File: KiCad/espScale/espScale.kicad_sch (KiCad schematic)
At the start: 7 parts, among them U1 NodeMCU1.0(ESP-12E), U2 3-wire_Load_Cell, U4 3-wire_Load_Cell, U6 HX711_Load_Cell_Amplifier

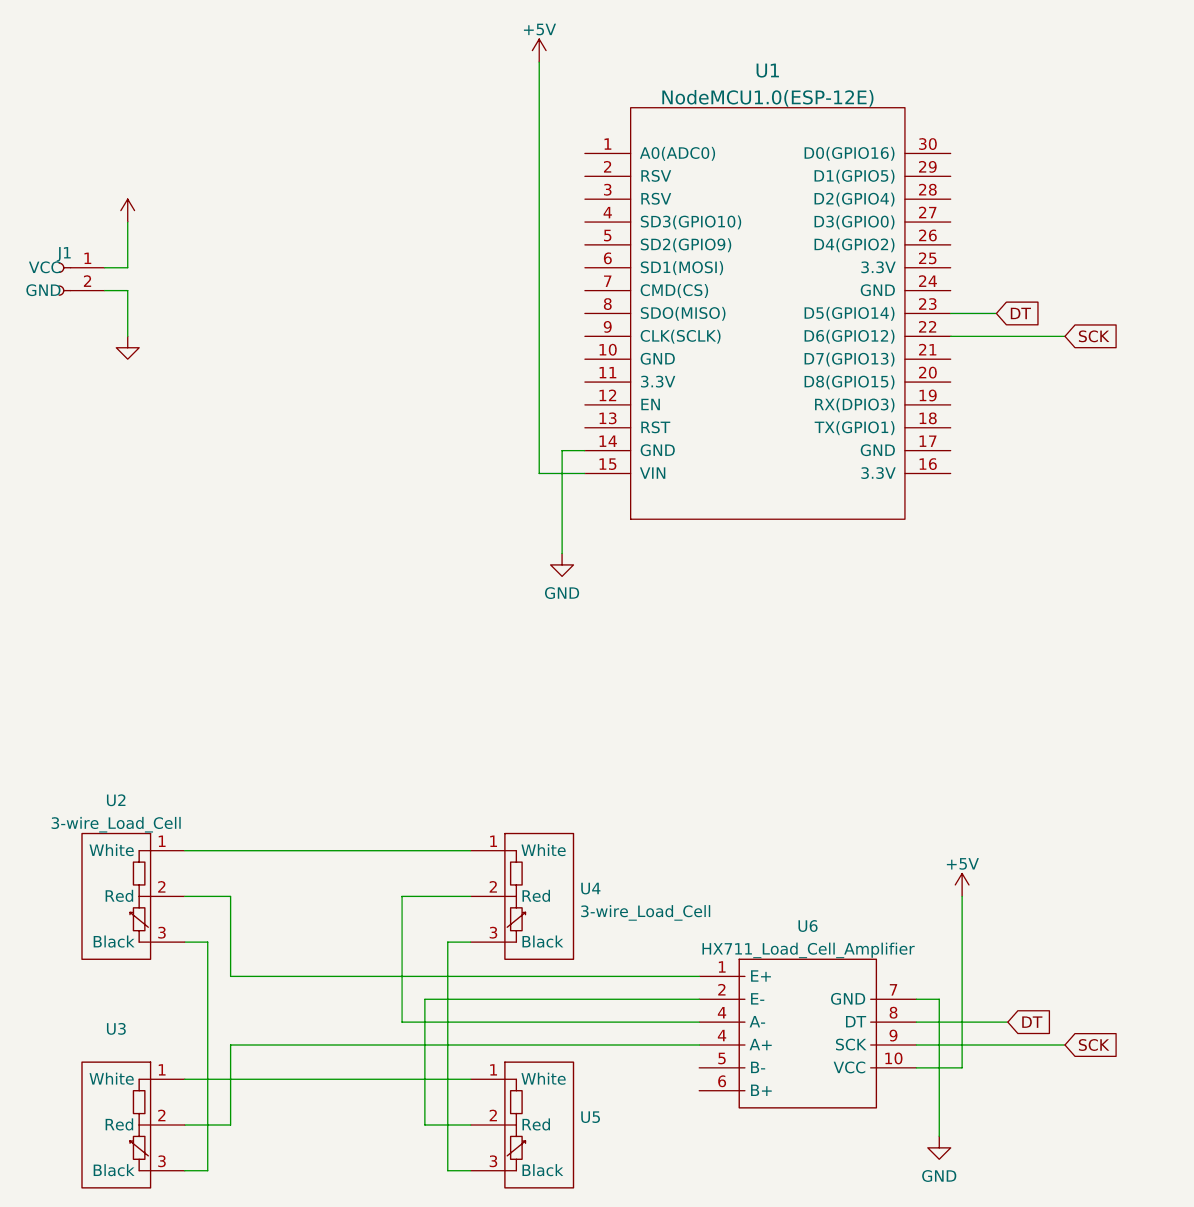
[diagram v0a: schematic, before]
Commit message: kicad
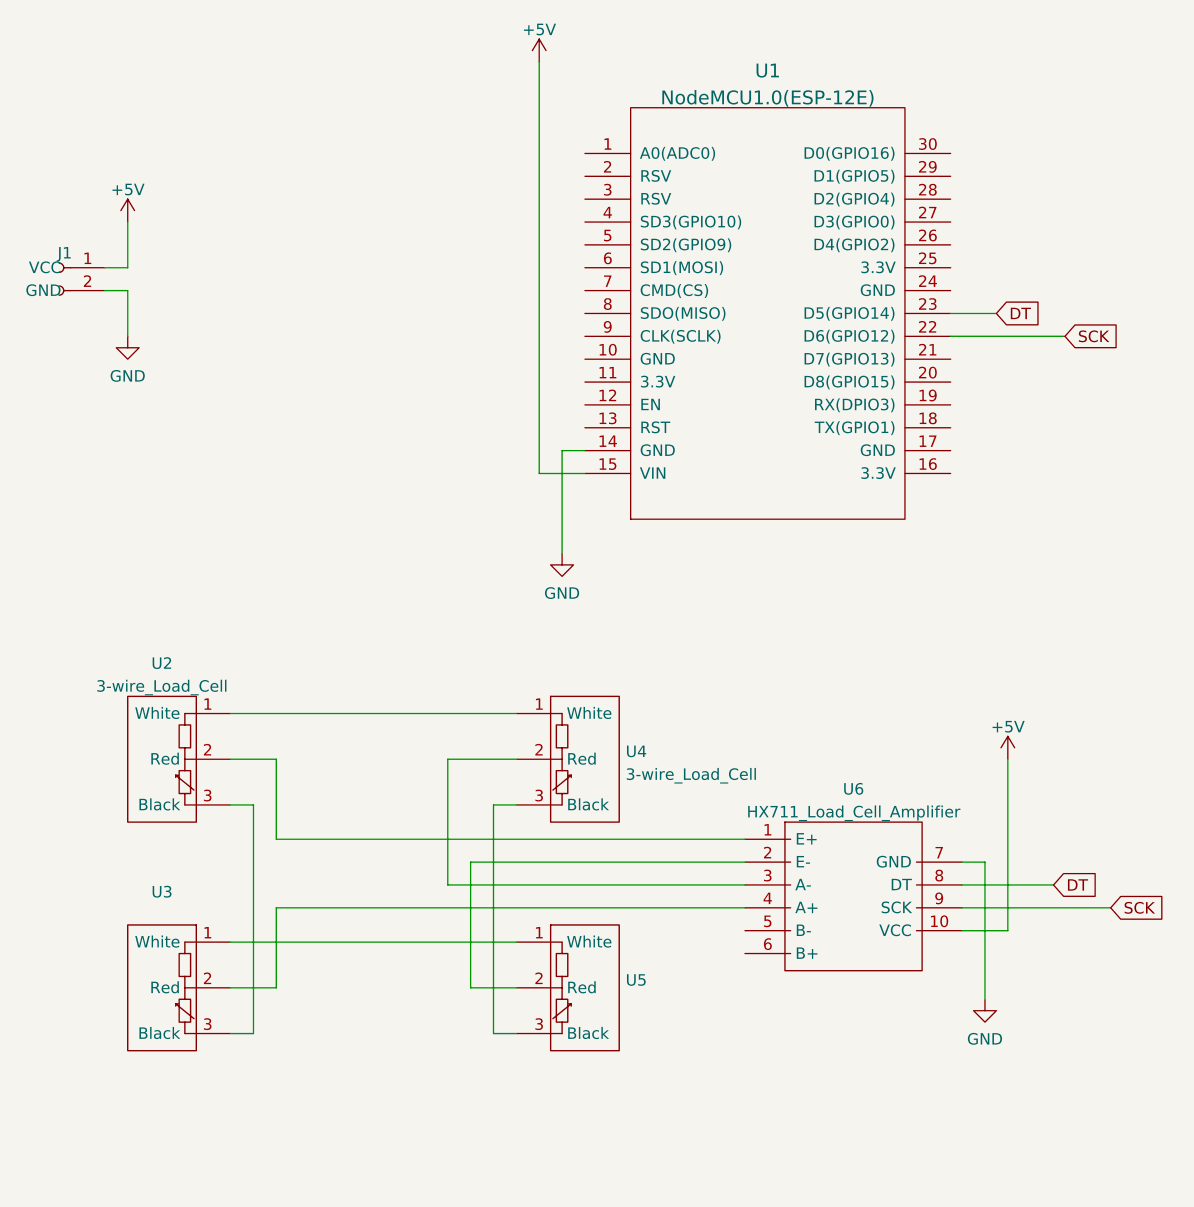
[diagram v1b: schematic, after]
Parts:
- J1: value (none) -> 2-pin_power_input_header; footprint (none) -> My_Headers:2-pin_power_input_header
- U2, U3, U4, U5: footprint (none) -> My_Headers:3-pin_load_cell_header_large
- U6: footprint (none) -> My_Parts:HX711 Load Cell Amplifier w_pinsockets_large
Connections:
- net at U4.2 (Red): now also U6.3 (A-); no longer U6.4 (A-)
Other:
- moved on the sheet: U2, U3, U4, U5, U6

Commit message: kicad page settings
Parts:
- U2, U3, U4, U5: footprint My_Headers:3-pin_load_cell_header_large -> My_Headers:3-pin JST load cell
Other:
- title: (none) -> espScale
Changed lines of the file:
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@@
 (kicad_sch (version 20211123) (generator eeschema)
   (paper "A4")
+  (title_block
+    (title "espScale")
+    (date "2022-09-18")
+    (rev "0.1")
+  )
   (wire (pts (xy 184.15 127) (xy 189.23 127))
     (stroke (width 0) (type default) (color 0 0 0 0))
@@
       (effects (font (size 1.27 1.27)) (justify left))
     )
-    (property "Footprint" "My_Headers:3-pin_load_cell_header_large" (id 2) (at 139.319 124.841 0)
+    (property "Footprint" "My_Headers:3-pin JST load cell" (id 2) (at 139.319 124.841 0)
       (effects (font (size 1.27 1.27)) hide)
     )
@@
     (property "Reference" "U2" (id 0) (at 95.25 97.316 0))
     (property "Value" "3-wire_Load_Cell" (id 1) (at 95.25 99.8529 0))
-    (property "Footprint" "My_Headers:3-pin_load_cell_header_large" (id 2) (at 98.171 99.441 0)
+    (property "Footprint" "My_Headers:3-pin JST load cell" (id 2) (at 98.171 99.441 0)
       (effects (font (size 1.27 1.27)) hide)
     )
@@
       (effects (font (size 1.27 1.27)) (justify left))
     )
-    (property "Footprint" "My_Headers:3-pin_load_cell_header_large" (id 2) (at 139.319 99.441 0)
+    (property "Footprint" "My_Headers:3-pin JST load cell" (id 2) (at 139.319 99.441 0)
       (effects (font (size 1.27 1.27)) hide)
     )
@@
     (property "Reference" "U3" (id 0) (at 95.25 122.716 0))
     (property "Value" "~" (id 1) (at 95.25 125.2529 0))
-    (property "Footprint" "My_Headers:3-pin_load_cell_header_large" (id 2) (at 98.171 124.841 0)
+    (property "Footprint" "My_Headers:3-pin JST load cell" (id 2) (at 98.171 124.841 0)
       (effects (font (size 1.27 1.27)) hide)
     )
@@
     )
     (path "/8af7217e-6b6b-49c7-a1b8-be8a38ecb040"
-      (reference "U2") (unit 1) (value "3-wire_Load_Cell") (footprint "My_Headers:3-pin_load_cell_header_large")
+      (reference "U2") (unit 1) (value "3-wire_Load_Cell") (footprint "My_Headers:3-pin JST load cell")
     )
     (path "/d6d827e1-8037-4a64-9433-b930cfff7250"
-      (reference "U3") (unit 1) (value "~") (footprint "My_Headers:3-pin_load_cell_header_large")
+      (reference "U3") (unit 1) (value "~") (footprint "My_Headers:3-pin JST load cell")
     )
     (path "/bad23df6-f465-434f-8740-c4824bad6534"
-      (reference "U4") (unit 1) (value "3-wire_Load_Cell") (footprint "My_Headers:3-pin_load_cell_header_large")
+      (reference "U4") (unit 1) (value "3-wire_Load_Cell") (footprint "My_Headers:3-pin JST load cell")
     )
     (path "/3209d3a7-a6c2-49ab-93de-4f7ab80f7cda"
-      (reference "U5") (unit 1) (value "~") (footprint "My_Headers:3-pin_load_cell_header_large")
+      (reference "U5") (unit 1) (value "~") (footprint "My_Headers:3-pin JST load cell")
     )
     (path "/3c667cba-91d1-4464-8b34-8c6b7fcac30a"
